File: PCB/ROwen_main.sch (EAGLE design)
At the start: 107 parts, among them CON1 MLW06_90°, CON2 MLW14_90°, CON3 S1G4_JUMP, CON4 S1G4_JUMP, CON5 MINI-USB-UX60-MB-5ST, CON6 S1G6_JUMP, IC1 STM32F042C, Q1 N-HEXFET-2D_SOT232-IRLL014N, SW1 P-B1720, SW2 P-B1720, SW3 P-B1720, SW4 P-B1720, X1 HC49

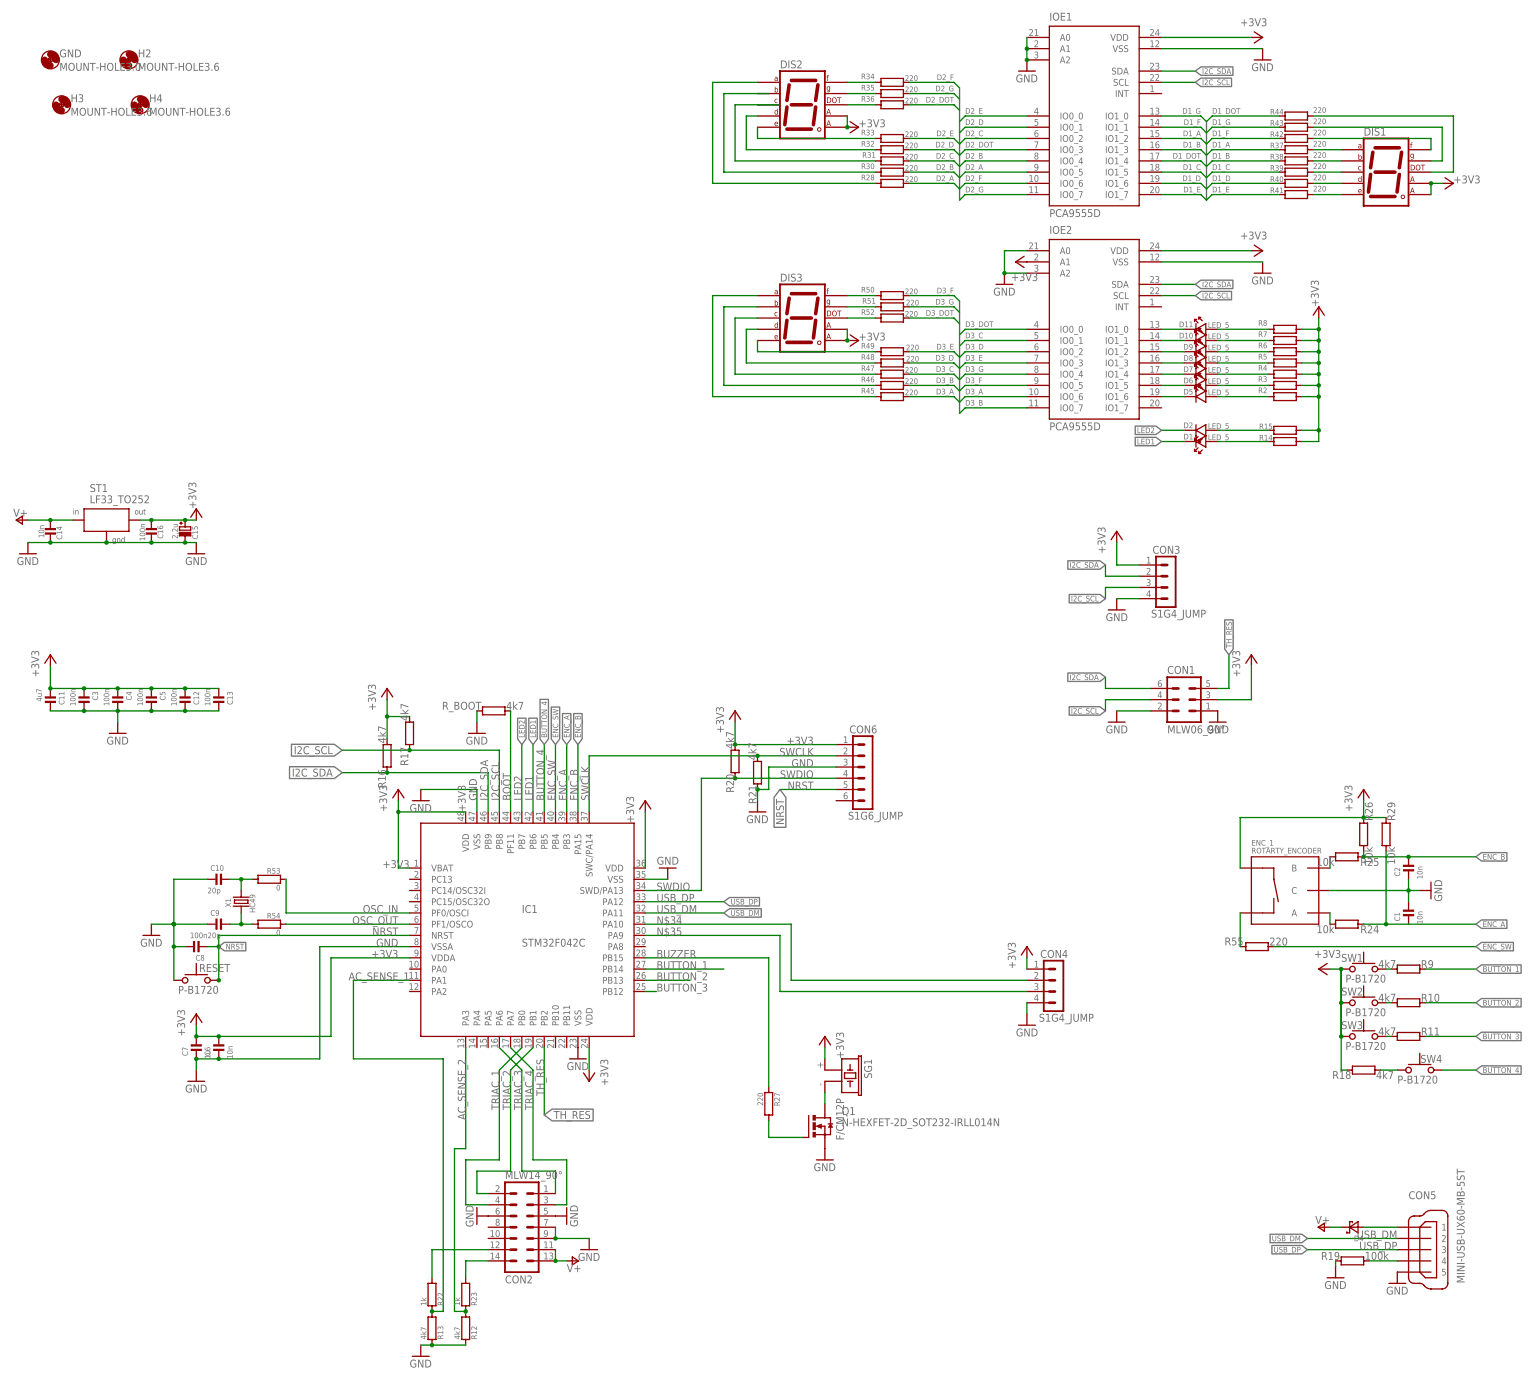
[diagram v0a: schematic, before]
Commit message: small PCB updates
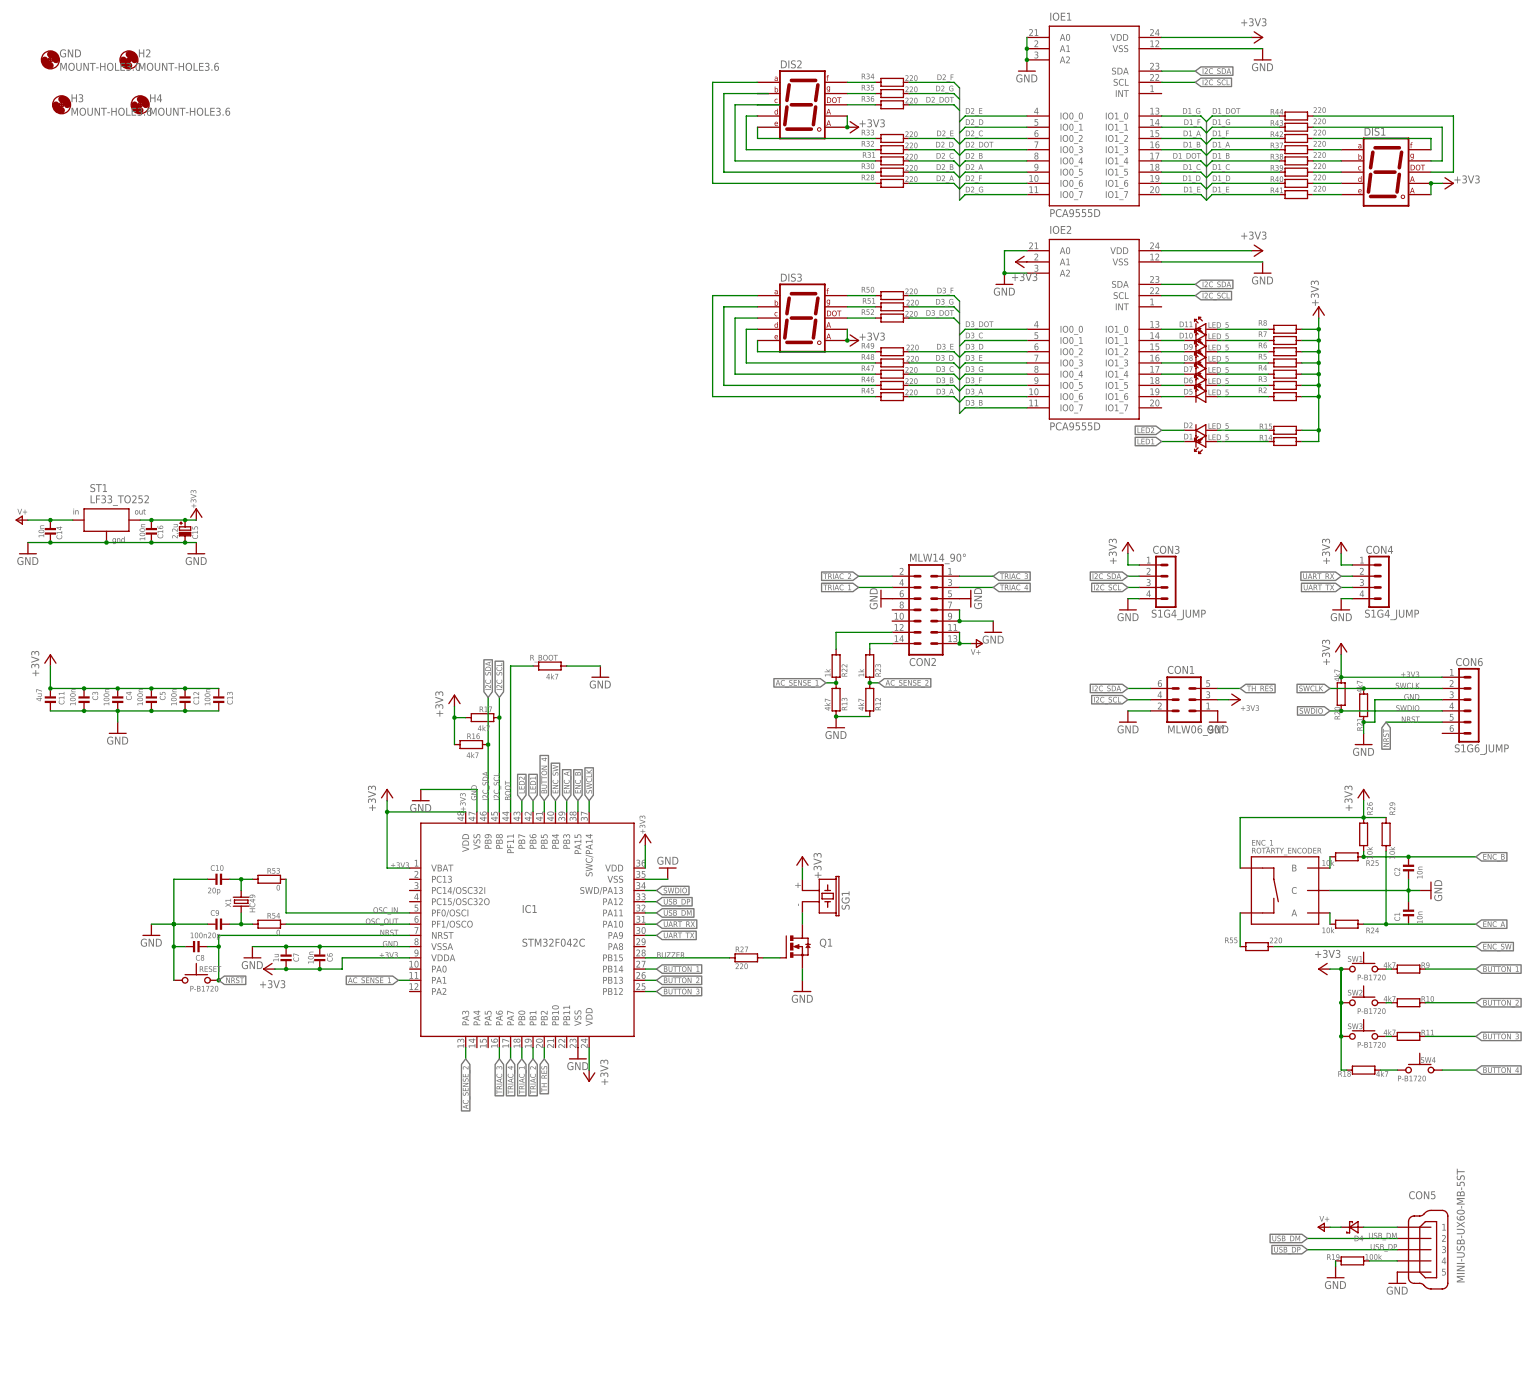
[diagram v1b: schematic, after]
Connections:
- net N$34 renamed UART_RX
- net N$35 renamed UART_TX
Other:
- note removed: "ap2204"
- moved on the sheet: C6, C7, CON2, CON4, CON6, Q1, R12, R13, R16, R17, R20, R21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
